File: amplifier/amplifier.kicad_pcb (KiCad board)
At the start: 2 copper layers, 54 x 46.8 mm, 20 parts, among them J1 INPUT, J3 POWER IN, Q1 TIP41, Q2 TIP42, U1 LM833

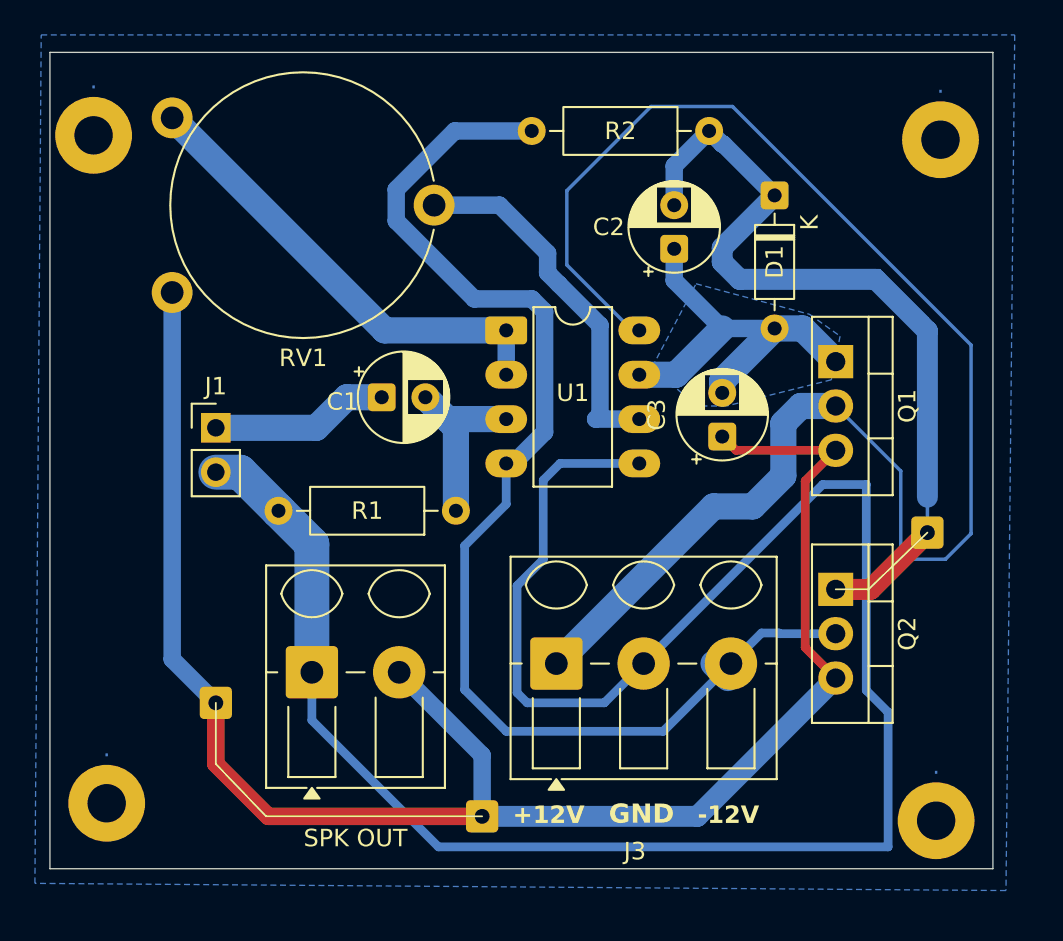
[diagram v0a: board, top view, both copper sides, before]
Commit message: Added HP@DESKTOP-614QREO MINGW64 ~/Documents/KICAD Project (main) $
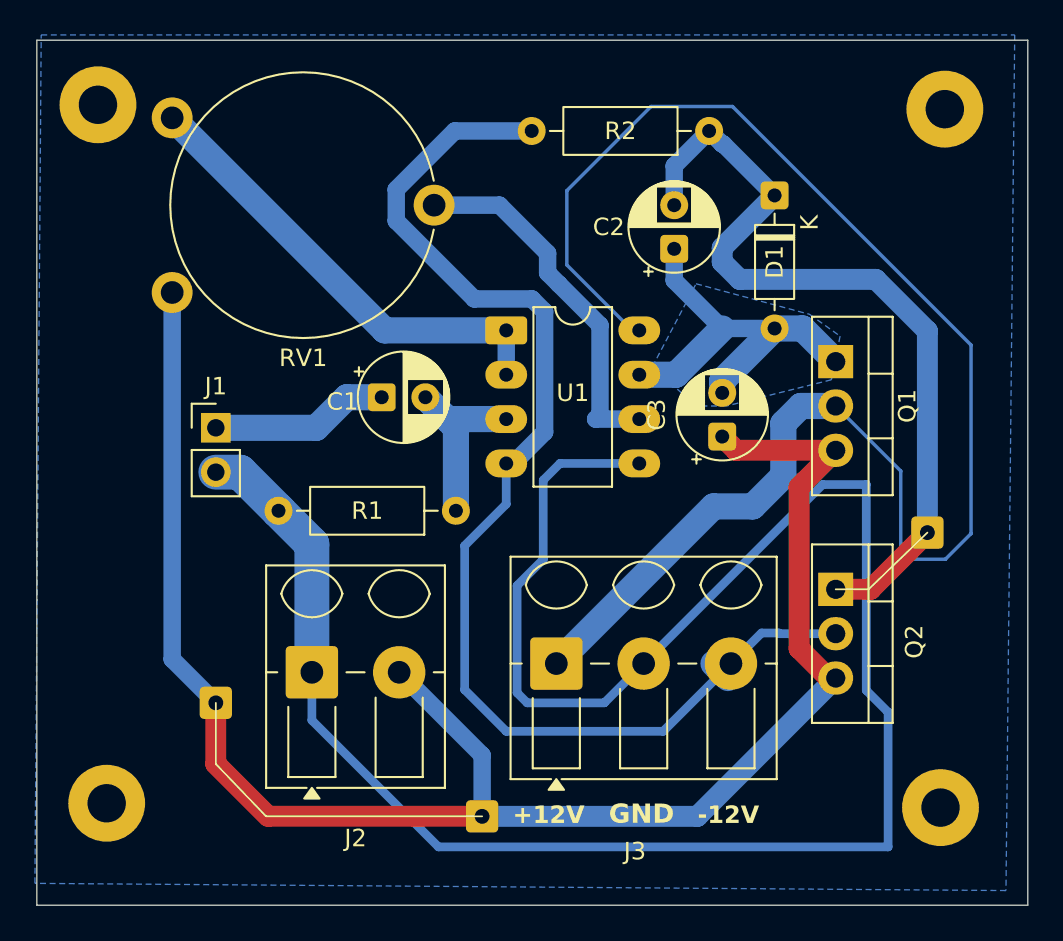
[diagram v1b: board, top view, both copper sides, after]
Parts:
- J2: renamed from SPK OUT
- moved . 1.77 mm to (95.2, 79.5)
- moved . 1.77 mm to (46.8, 79.2)
- moved . 0.79 mm to (95.0, 119.5)
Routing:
- net Net-(D1-K): track 70.9 -> 46.9 mm
- net Net-(J2-Pin_2): track 99.6 -> 100.1 mm
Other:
- board size 54 x 46.8 mm -> 56.7 x 49.5 mm
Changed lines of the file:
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@@
 		(sheetname "/")
 		(sheetfile "amplifier.kicad_sch")
+		(units
+			(unit
+				(name "A")
+				(pins "1" "2")
+			)
+		)
 		(attr through_hole)
 		(duplicate_pad_numbers_are_jumpers no)
@@
 	(footprint "MountingHole:MountingHole_2.2mm_M2_Pad"
 		(layer "F.Cu")
-		(at 95 81.25)
+		(at 95.25 79.5)
 		(descr "Mounting Hole 2.2mm, M2, generated by kicad-footprint-generator mountinghole.py")
 		(tags "mountinghole M2")
@@
 			(at 0 -3.15 0)
 			(layer "B.Cu")
+			(hide yes)
 			(effects
 				(font
@@
 		(sheetname "/")
 		(sheetfile "amplifier.kicad_sch")
+		(units
+			(unit
+				(name "A")
+				(pins "1" "2")
+			)
+		)
 		(attr through_hole)
 		(duplicate_pad_numbers_are_jumpers no)
@@
 			)
 		)
-		(property "Description" ""
+		(property "Description" "Trim-potentiometer, US symbol"
 			(at 0 0 0)
 			(layer "F.Fab")
@@
 		(sheetname "/")
 		(sheetfile "amplifier.kicad_sch")
+		(units
+			(unit
+				(name "A")
+				(pins "1" "3" "2")
+			)
+		)
 		(attr through_hole)
 		(duplicate_pad_numbers_are_jumpers no)
@@
 		(descr "Terminal block Altech AK300, 45Degree (cable under 45degree), 2 pins, pitch 5mm, size 10x12.5mm, drill diameter 1.3mm, pad diameter 3mm, https://www.altechcorp.com/PDFS/PCBMETRC.PDF#page=5, generated with kicad-footprint-generator TerminalBlock_Altech")
 		(tags "THT Terminal block Altech AK300 45Degree pitch 5mm size 10x12.5mm drill 1.3mm pad 3mm")
-		(property "Reference" "SPK OUT"
+		(property "Reference" "J2"
 			(at 2.5 9.5 0)
 			(layer "F.SilkS")
@@
 		(sheetname "/")
 		(sheetfile "amplifier.kicad_sch")
+		(units
+			(unit
+				(name "A")
+				(pins "1" "2")
+			)
+		)
 		(attr through_hole)
 		(duplicate_pad_numbers_are_jumpers no)
@@
 		(sheetname "/")
 		(sheetfile "amplifier.kicad_sch")
+		(units
+			(unit
+				(name "A")
+				(pins "1" "2")
+			)
+		)
 		(attr through_hole)
 		(duplicate_pad_numbers_are_jumpers no)
@@
 		(sheetname "/")
 		(sheetfile "amplifier.kicad_sch")
+		(units
+			(unit
+				(name "A")
+				(pins "1" "2" "3")
+			)
+		)
 		(attr through_hole)
 		(duplicate_pad_numbers_are_jumpers no)
@@
 			(at 0 -3.15 0)
 			(layer "B.Cu")
+			(hide yes)
 			(effects
 				(font
@@
 		(sheetname "/")
 		(sheetfile "amplifier.kicad_sch")
+		(units
+			(unit
+				(name "A")
+				(pins "1" "2")
+			)
+		)
 		(attr through_hole)
 		(duplicate_pad_numbers_are_jumpers no)
@@
 		(sheetname "/")
 		(sheetfile "amplifier.kicad_sch")
+		(units
+			(unit
+				(name "A")
+				(pins "1" "2" "3")
+			)
+		)
 		(attr through_hole)
 		(duplicate_pad_numbers_are_jumpers no)
@@
 	(footprint "MountingHole:MountingHole_2.2mm_M2_Pad"
 		(layer "F.Cu")
-		(at 46.5 81)
+		(at 46.75 79.25)
 		(descr "Mounting Hole 2.2mm, M2, generated by kicad-footprint-generator mountinghole.py")
 		(tags "mountinghole M2")
@@
 			(at 0 -3.15 0)
 			(layer "B.Cu")
+			(hide yes)
 			(effects
 				(font
@@
 	(footprint "MountingHole:MountingHole_2.2mm_M2_Pad"
 		(layer "F.Cu")
-		(at 94.75 120.25)
+		(at 95 119.5)
 		(descr "Mounting Hole 2.2mm, M2, generated by kicad-footprint-generator mountinghole.py")
 		(tags "mountinghole M2")
@@
 			(at 0 -3.15 0)
 			(layer "B.Cu")
+			(hide yes)
 			(effects
 				(font
@@
 		(sheetname "/")
 		(sheetfile "amplifier.kicad_sch")
+		(units
+			(unit
+				(name "A")
+				(pins "1" "2")
+			)
+		)
 		(attr through_hole)
 		(duplicate_pad_numbers_are_jumpers no)
@@
 		(tags "TO-220-3 Vertical RM 2.54mm")
 		(property "Reference" "Q2"
-			(at 2.54 -4.1 90)
+			(at 3 -4.5 90)
 			(layer "F.SilkS")
 			(effects
@@
 		(sheetname "/")
 		(sheetfile "amplifier.kicad_sch")
+		(units
+			(unit
+				(name "A")
+				(pins "1" "2" "3")
+			)
+		)
 		(attr through_hole)
 		(duplicate_pad_numbers_are_jumpers no)
@@
 		(sheetname "/")
 		(sheetfile "amplifier.kicad_sch")
+		(units
+			(unit
+				(name "A")
+				(pins "1" "2")
+			)
+		)
 		(attr through_hole)
 		(duplicate_pad_numbers_are_jumpers no)
@@
 		(sheetname "/")
 		(sheetfile "amplifier.kicad_sch")
+		(units
+			(unit
+				(name "A")
+				(pins "3" "2" "1")
+			)
+			(unit
+				(name "B")
+				(pins "5" "6" "7")
+			)
+			(unit
+				(name "C")
+				(pins "8" "4")
+			)
+		)
 		(attr through_hole)
 		(duplicate_pad_numbers_are_jumpers no)
@@
 		(sheetname "/")
 		(sheetfile "amplifier.kicad_sch")
+		(units
+			(unit
+				(name "A")
+				(pins "1" "2")
+			)
+		)
 		(attr through_hole)
 		(duplicate_pad_numbers_are_jumpers no)
@@
 	)
 	(gr_rect
-		(start 44 76.25)
-		(end 98 123)
+		(start 43.25 75.553072)
+		(end 99.999999 125.089914)
 		(stroke
 			(width 0.05)
@@
 	)
 	(segment
-		(start 56.5 120)
-		(end 53.5 117)
-		(width 1)
+		(start 86.9 110.390173)
+		(end 86.9 101.14)
+		(width 1.2)
 		(layer "F.Cu")
 		(net "Net-(J2-Pin_2)")
 	)
 	(segment
-		(start 89 99.04)
-		(end 83.29 99.04)
-		(width 0.5)
+		(start 83.29 99.04)
+		(end 89 99.04)
+		(width 1.2)
 		(layer "F.Cu")
 		(net "Net-(J2-Pin_2)")
 	)
 	(segment
-		(start 83.29 99.04)
-		(end 82.5 98.25)
-		(width 0.5)
+		(start 86.9 101.14)
+		(end 87.25 100.79)
+		(width 1.2)
 		(layer "F.Cu")
 		(net "Net-(J2-Pin_2)")
 	)
 	(segment
-		(start 68.75 120)
-		(end 56.5 120)
-		(width 1)
+		(start 82.5 98.25)
+		(end 83.29 99.04)
+		(width 1.2)
 		(layer "F.Cu")
 		(net "Net-(J2-Pin_2)")
 	)
 	(segment
-		(start 87.25 110.33)
-		(end 87.25 100.79)
-		(width 0.5)
+		(start 89 112.08)
+		(end 88.589827 112.08)
+		(width 1.2)
 		(layer "F.Cu")
 		(net "Net-(J2-Pin_2)")
 	)
 	(segment
-		(start 89 112.08)
-		(end 87.25 110.33)
-		(width 0.5)
+		(start 56.5 120)
+		(end 68.75 120)
+		(width 1.2)
+		(layer "F.Cu")
+		(net "Net-(J2-Pin_2)")
+	)
+	(segment
+		(start 53.5 117)
+		(end 56.5 120)
+		(width 1.2)
 		(layer "F.Cu")
 		(net "Net-(J2-Pin_2)")
@@
 		(start 87.25 100.79)
 		(end 89 99.04)
-		(width 0.5)
+		(width 1.2)
 		(layer "F.Cu")
 		(net "Net-(J2-Pin_2)")
 	)
 	(segment
-		(start 53.5 117)
-		(end 53.5 113.5)
-		(width 1)
+		(start 88.589827 112.08)
+		(end 86.9 110.390173)
+		(width 1.2)
+		(layer "F.Cu")
+		(net "Net-(J2-Pin_2)")
+	)
+	(segment
+		(start 53.5 113.5)
+		(end 53.5 117)
+		(width 1.2)
 		(layer "F.Cu")
 		(net "Net-(J2-Pin_2)")
@@
 		(end 73.6 88.42)
 		(width 0.2)
+		(locked yes)
 		(layer "B.Cu")
 		(net "+12V")
@@
 	)
 	(segment
-		(start 94.25 91.5)
-		(end 91.5 88.75)
-		(width 0.2)
-		(layer "B.Cu")
-		(net "Net-(D1-K)")
-	)
-	(segment
 		(start 85.5 84.44)
 		(end 82.5 87.44)
@@
 	(segment
 		(start 94.25 92.207107)
-		(end 94.25 101.725)
+		(end 94.25 103.75)
 		(width 1.2)
 		(layer "B.Cu")
@@
 	)
 	(segment
-		(start 91.5 88.75)
-		(end 83.25 88.75)
-		(width 0.2)
-		(layer "B.Cu")
-		(net "Net-(D1-K)")
-	)
-	(segment
-		(start 83.25 88.75)
-		(end 82.5 88)
-		(width 0.2)
-		(layer "B.Cu")
-		(net "Net-(D1-K)")
-	)
-	(segment
 		(start 83.5 89.25)
 		(end 91.292893 89.25)
@@
 		(layer "B.Cu")
 		(net "Net-(D1-K)")
-	)
-	(segment
-		(start 82.5 88)
-		(end 82.5 87.44)
-		(width 0.2)
-		(layer "B.Cu")
-		(net "Net-(D1-K)")
-	)
-	(segment
-		(start 94.25 103.75)
-		(end 94.25 91.5)
-		(width 0.2)
-		(layer "B.Cu")
-		(net "Net-(D1-K)")
